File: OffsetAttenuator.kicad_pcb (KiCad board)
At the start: 2 copper layers, 17 parts, among them J1 Conn_Coaxial, J2 Conn_Coaxial, SW1 POWER, SW2 BYPASS, U1 L7805, Y1 ECS-2100AX-040

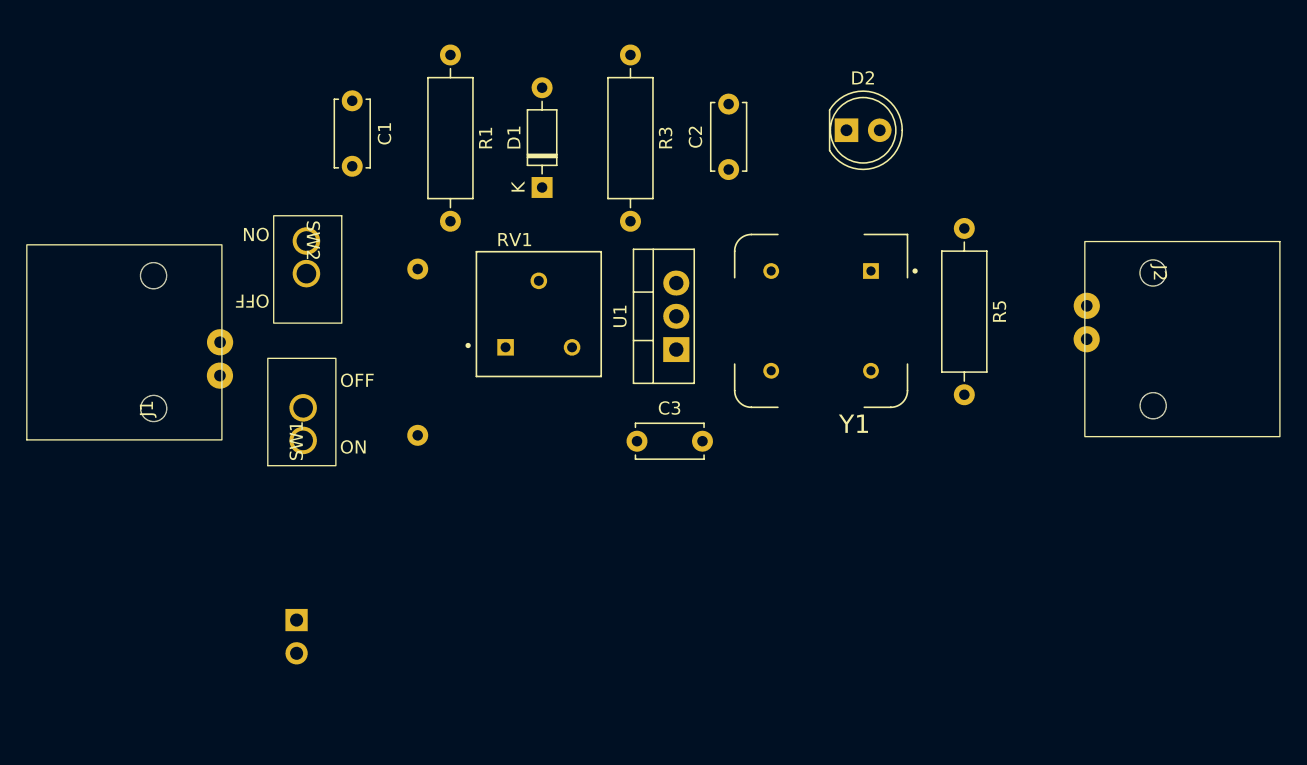
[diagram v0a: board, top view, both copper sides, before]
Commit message: more layout
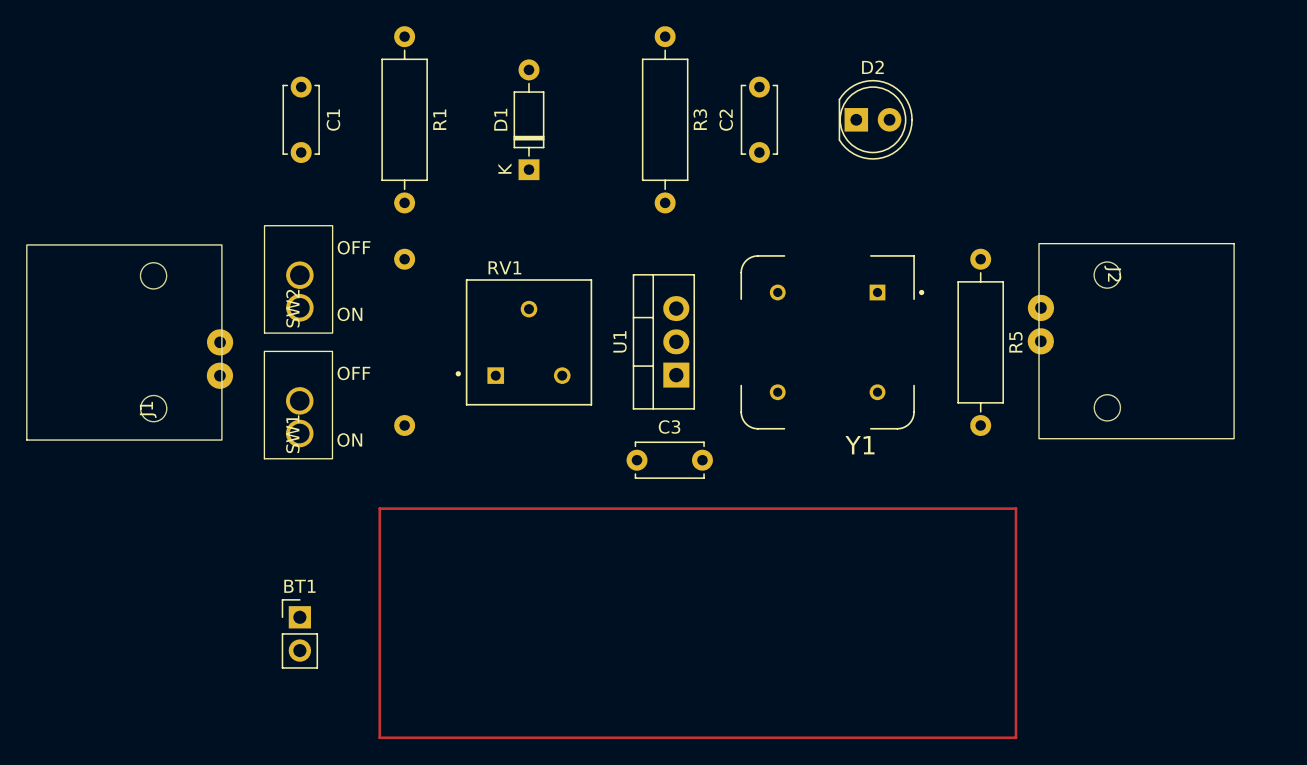
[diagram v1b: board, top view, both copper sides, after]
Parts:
- BT1: moved to F.Cu
- moved SW2 5.20 mm to (53.0, 48.9), turned to 90 degrees
- moved C1 4.04 mm to (53.1, 32.0)
- moved R1 3.77 mm to (61.0, 28.1)
- moved J2 3.50 mm to (114.7, 46.4)
- moved R3 3.00 mm to (80.9, 28.1)
- moved C2 2.69 mm to (88.1, 37.0)
- moved R5 2.66 mm to (105.0, 45.1)
- moved RV1 2.29 mm to (70.5, 51.5)
- moved U1 1.95 mm to (81.8, 54.0)
- moved Y1 1.71 mm to (93.3, 51.5)
- moved D1 1.69 mm to (70.5, 38.3)
- moved C3 1.45 mm to (78.8, 60.5)
- moved R4 1.25 mm to (61.0, 45.1)
- moved D2 1.10 mm to (95.5, 34.5)
- moved SW1 0.59 mm to (53.0, 58.5)
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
